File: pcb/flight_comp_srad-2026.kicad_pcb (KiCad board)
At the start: 4 copper layers, 70 x 40 mm, 64 parts, among them J1 503398-1892, J3 USB_B_Micro, U1 IIM-20670, U2 NCP1117-3.3_SOT223, U3 RP2040, U4 ADXL375BCCZ-RL7, U5 MAX-M10M-00B, U6 W25Q128JVS, U7 XBP9B-DMSTB002, Y1 ABM8-272-T3

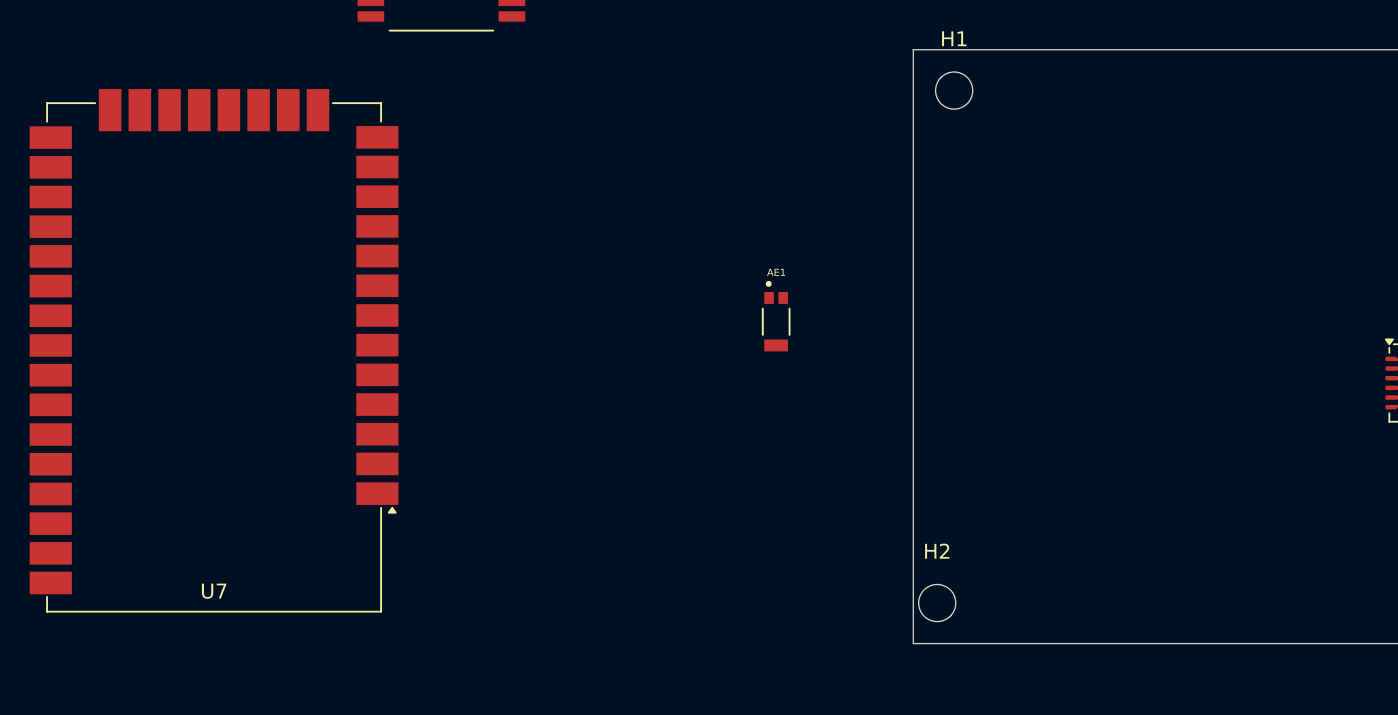
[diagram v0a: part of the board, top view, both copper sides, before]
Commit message: cosas del xbee
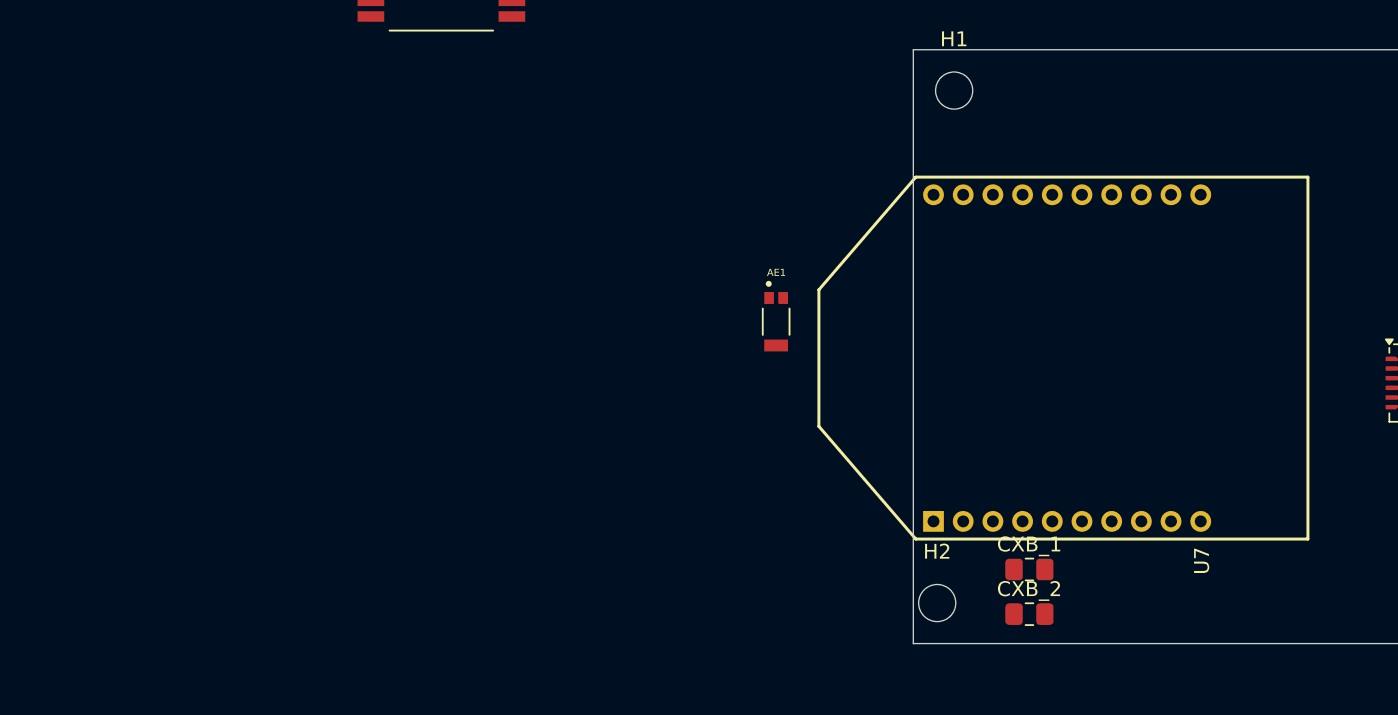
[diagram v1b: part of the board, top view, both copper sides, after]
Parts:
- added CXB_1: C, TCLib:C_0805, F.Cu at (159.0, 95.5)
- added CXB_2: C, TCLib:C_0805, F.Cu at (159.0, 98.5)
- U7: footprint RF_Module:Digi_XBee_SMT -> SRAD_fligh_comp2026:XBEEPRO
- moved U7 57.2 mm to (161.2, 81.2), turned to 90 degrees
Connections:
- RFLASH_1 pad 1: GND -> +3V3
- RI2C_1 pad 2: GND -> +3V3
- RI2C_2 pad 2: GND -> +3V3
- U3 pad 1: GND -> +3V3
- U6 pad 8: GND -> +3V3
- U7 pad 1: unconnected-(U7-VCC-Pad1) -> +3V3
- U7 pad 10: unconnected-(U7-GND-Pad10) -> GND
- U7 pad 2: unconnected-(U7-DOUT/DIO13-Pad2) -> /UART_Rx
- U7 pad 3: unconnected-(U7-DIN/NCONFIG/DIO14-Pad3) -> /UART_Tx
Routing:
- net +3V3: track 7.04 -> 16.7 mm, vias 0 -> 3
- net GND: track 13.0 -> 3.32 mm, vias 20 -> 17
